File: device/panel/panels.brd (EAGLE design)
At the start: 133 x 77 mm, 0 parts

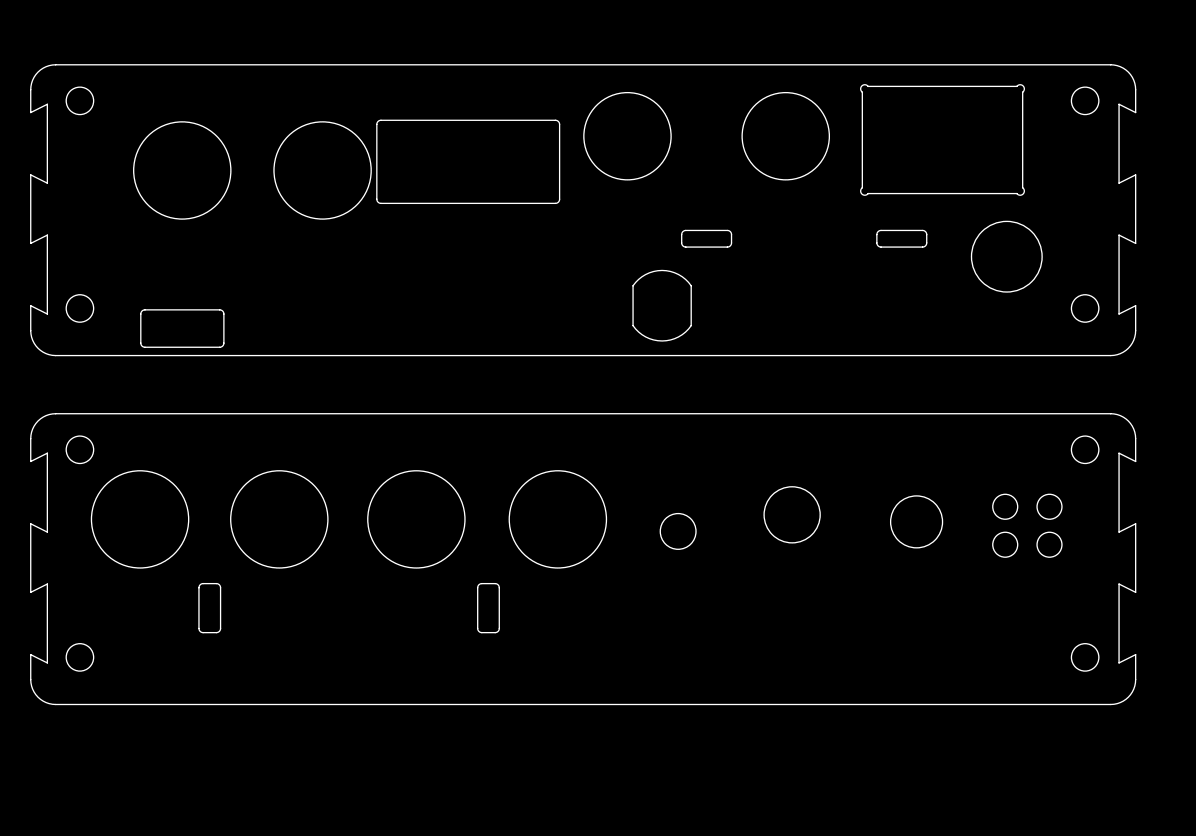
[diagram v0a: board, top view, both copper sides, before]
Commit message: More panel work.
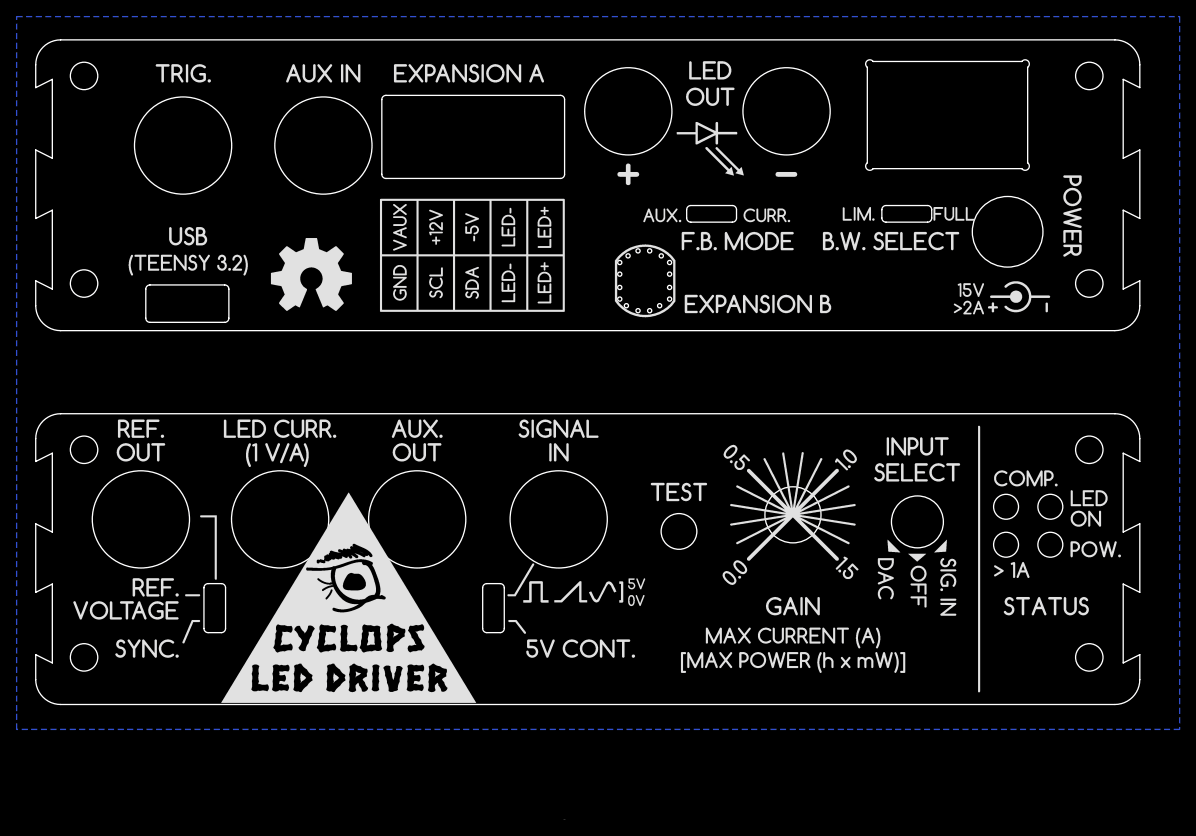
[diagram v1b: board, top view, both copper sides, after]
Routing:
- added copper zone on layer 16, net S$1
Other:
- board size 133 x 77 mm -> 132.9 x 80 mm
